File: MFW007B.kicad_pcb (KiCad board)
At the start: 4 copper layers, 84 x 42 mm, 96 parts, among them J1 Conn_01x04, J2 Conn_02x07, J3 4P JST-SH, J4 Conn_02x03, SW2 SW_Push, SW3 SW_Push, SW4 SW_Push, U1 24AA02-OT, U2 W5500, U3 STM32F103C8T6, U4 XC6206P332MR-G-SOT23, Y1 25MHz, Y2 8MHz, Y3 32.768KHz

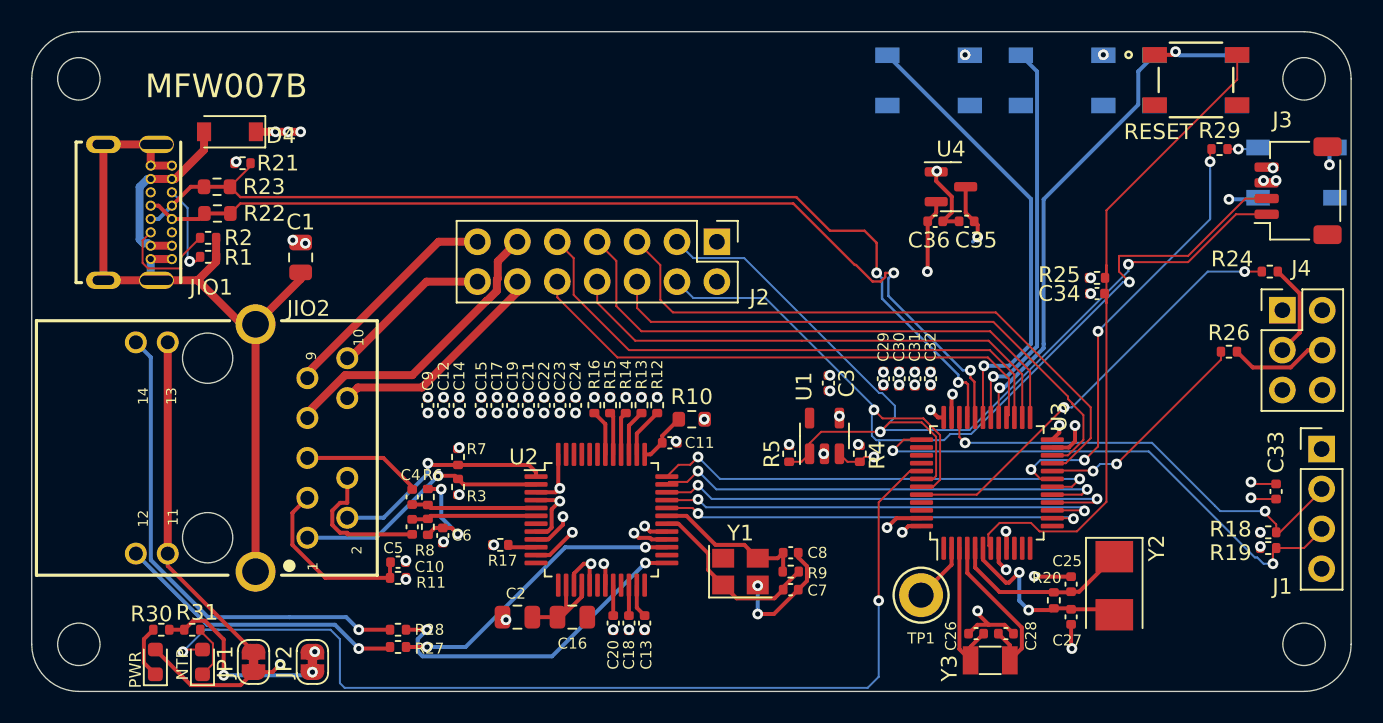
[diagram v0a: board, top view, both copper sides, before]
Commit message: fix DRC
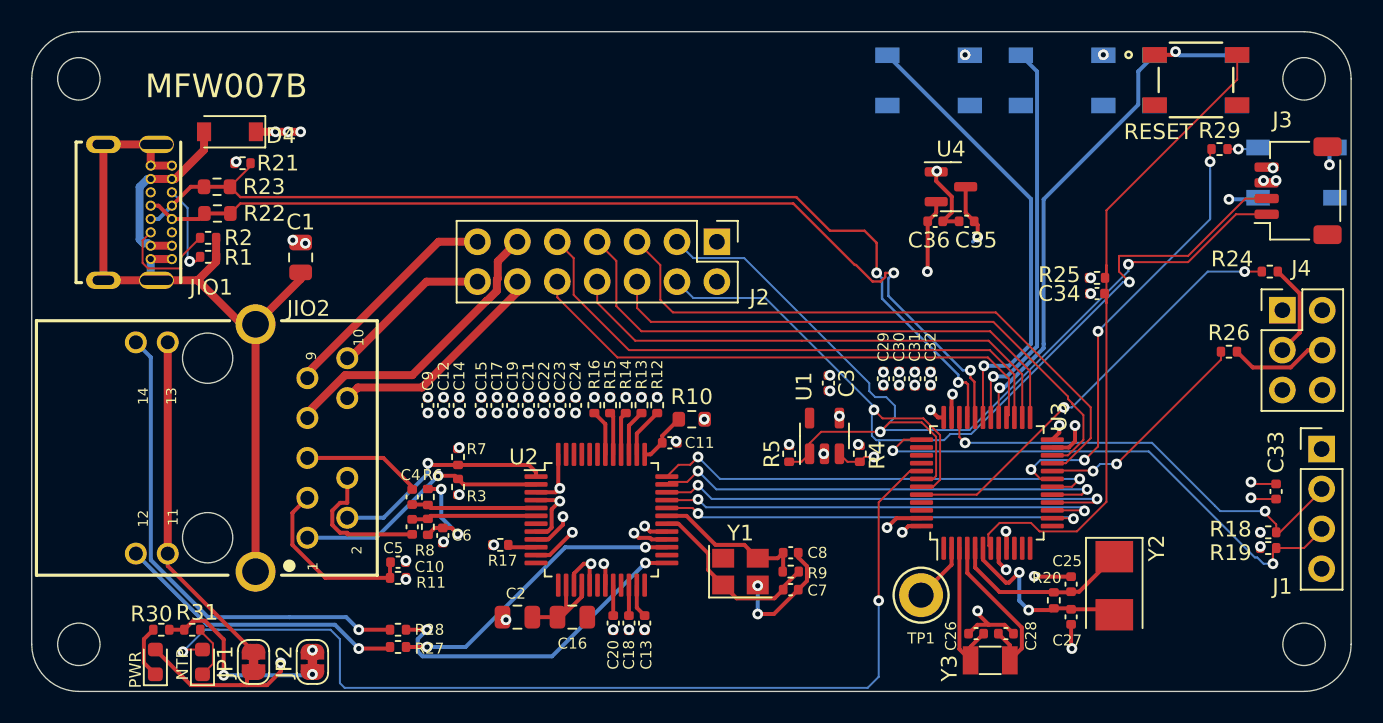
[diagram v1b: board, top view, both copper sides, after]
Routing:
- net +3V3: track 33.9 -> 35.3 mm
